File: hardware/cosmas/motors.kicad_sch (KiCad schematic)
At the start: 6 parts, among them J3 MOTORA, J4 MOTORB, J5 DRIVER-POWER, J6 MOTOR-CONTROL, J7 MOT_A, J8 MOT_A

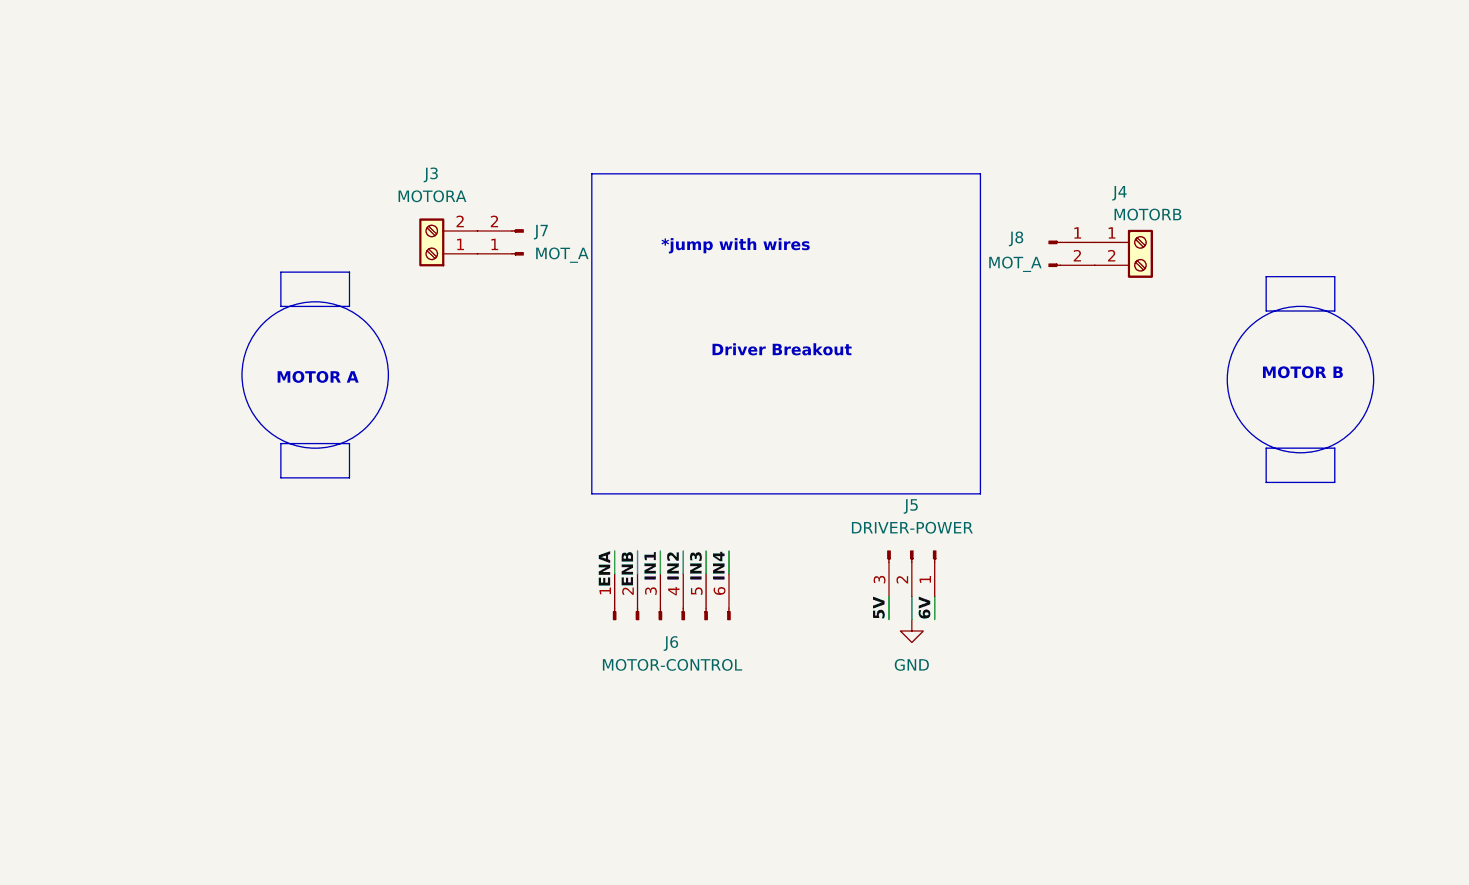
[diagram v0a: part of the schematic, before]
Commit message: adds OBC PCB
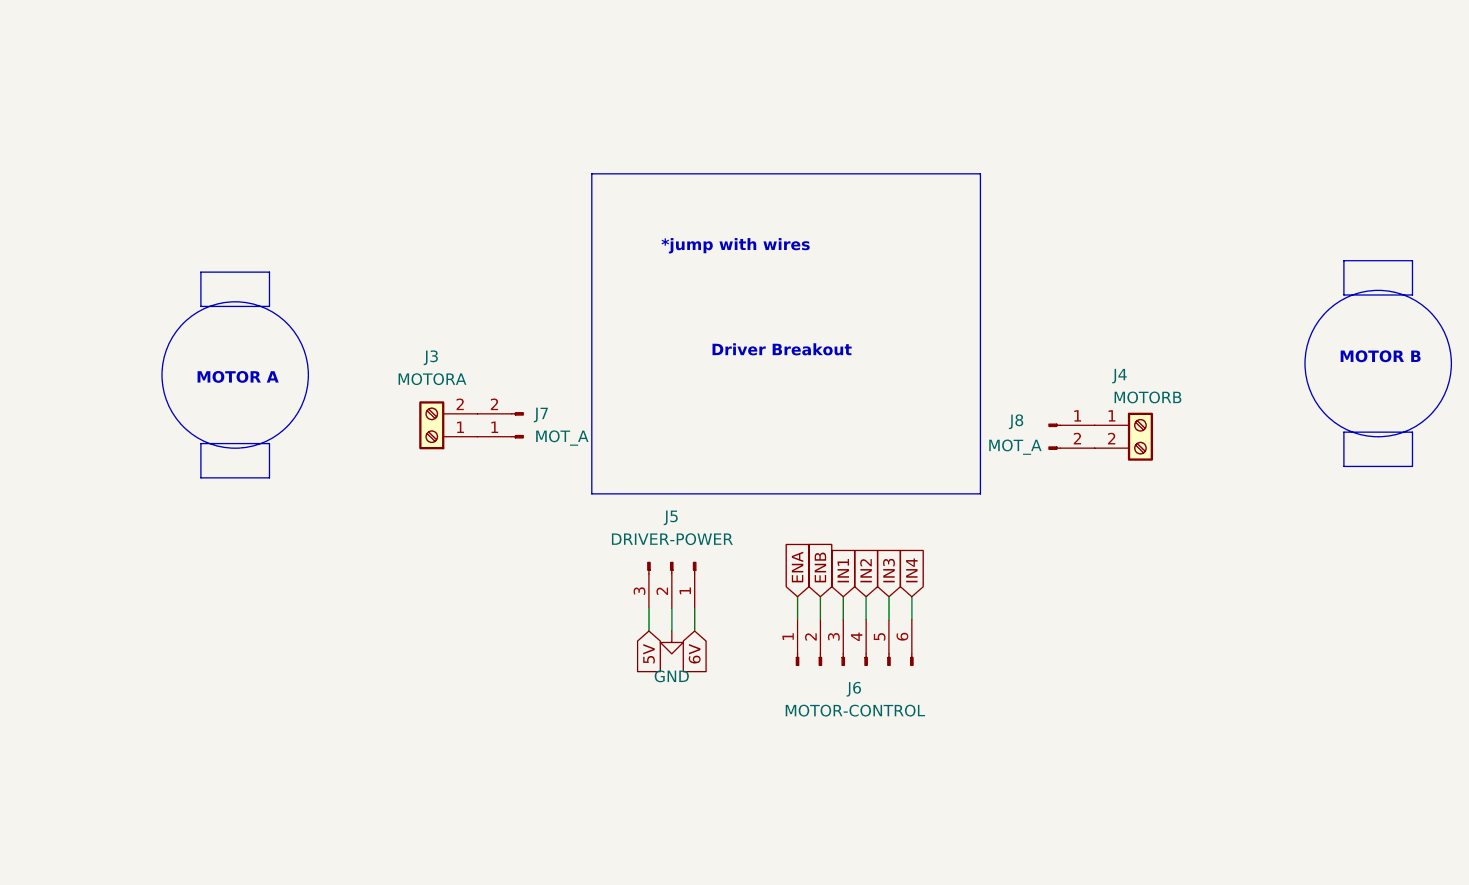
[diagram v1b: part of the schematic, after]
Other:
- moved on the sheet: J3, J4, J5, J6, J7, J8
